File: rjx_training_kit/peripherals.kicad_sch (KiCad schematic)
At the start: 31 parts, among them Q7 BC817, Q8 BC817, SW3 SW_Push, U2 BME280, U3 DS3231M, U5 LIS3DH, U8 BQ27441-G1

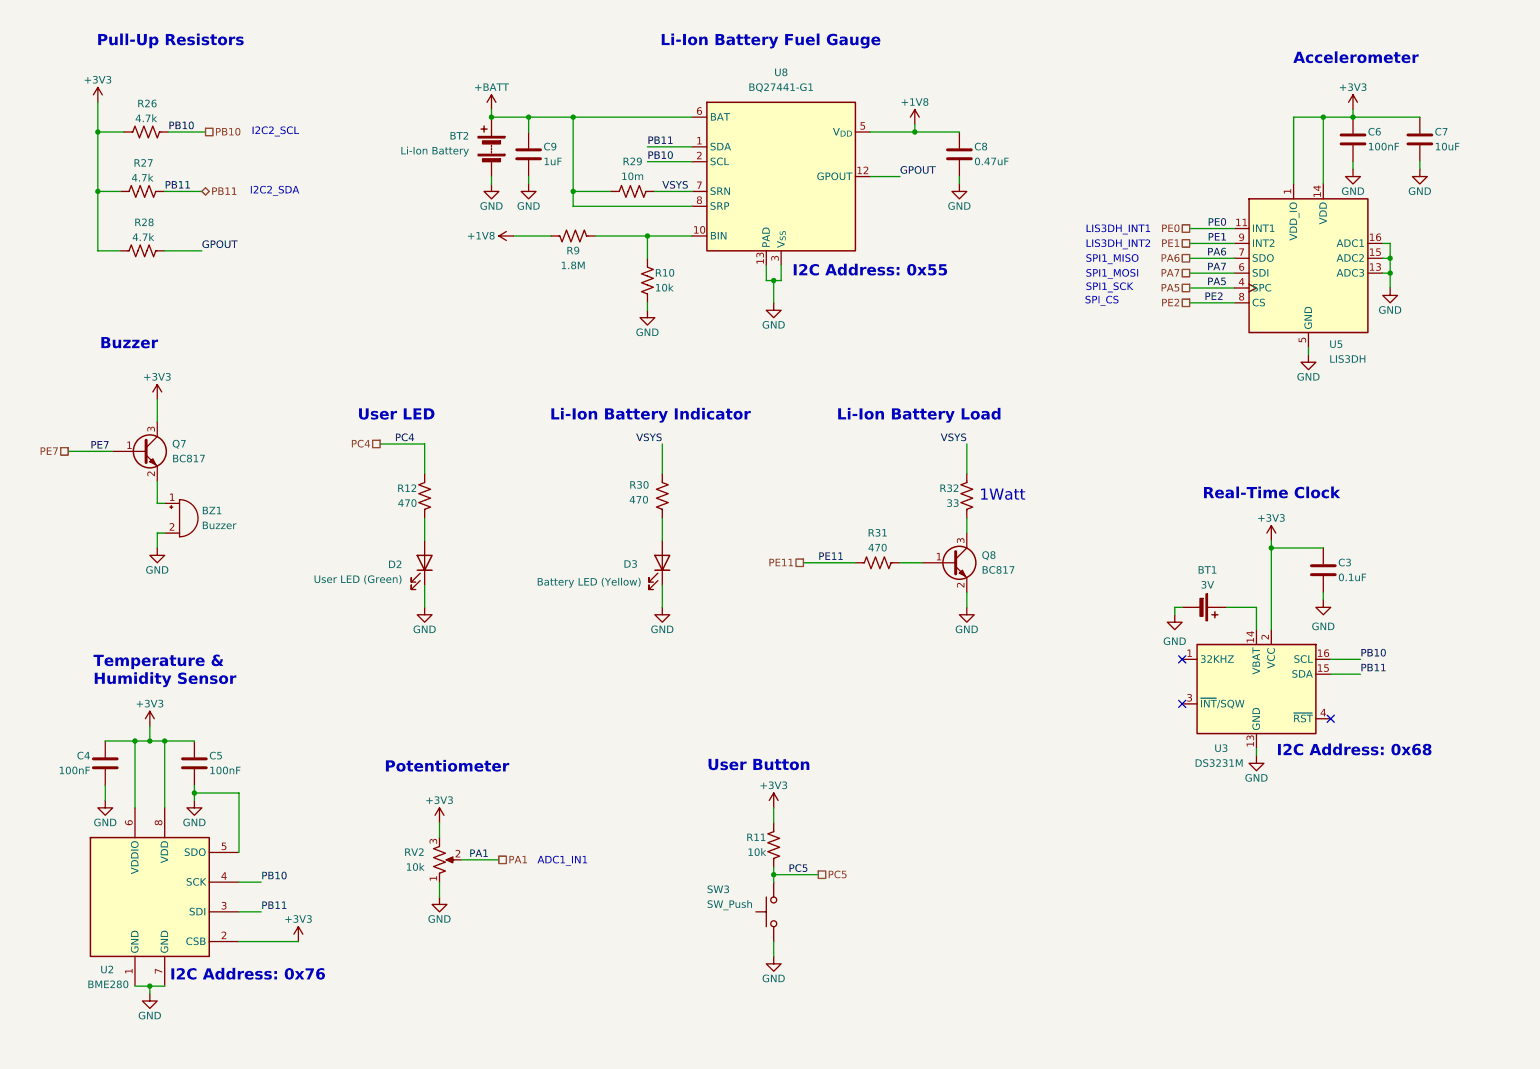
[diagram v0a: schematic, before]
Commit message: Update
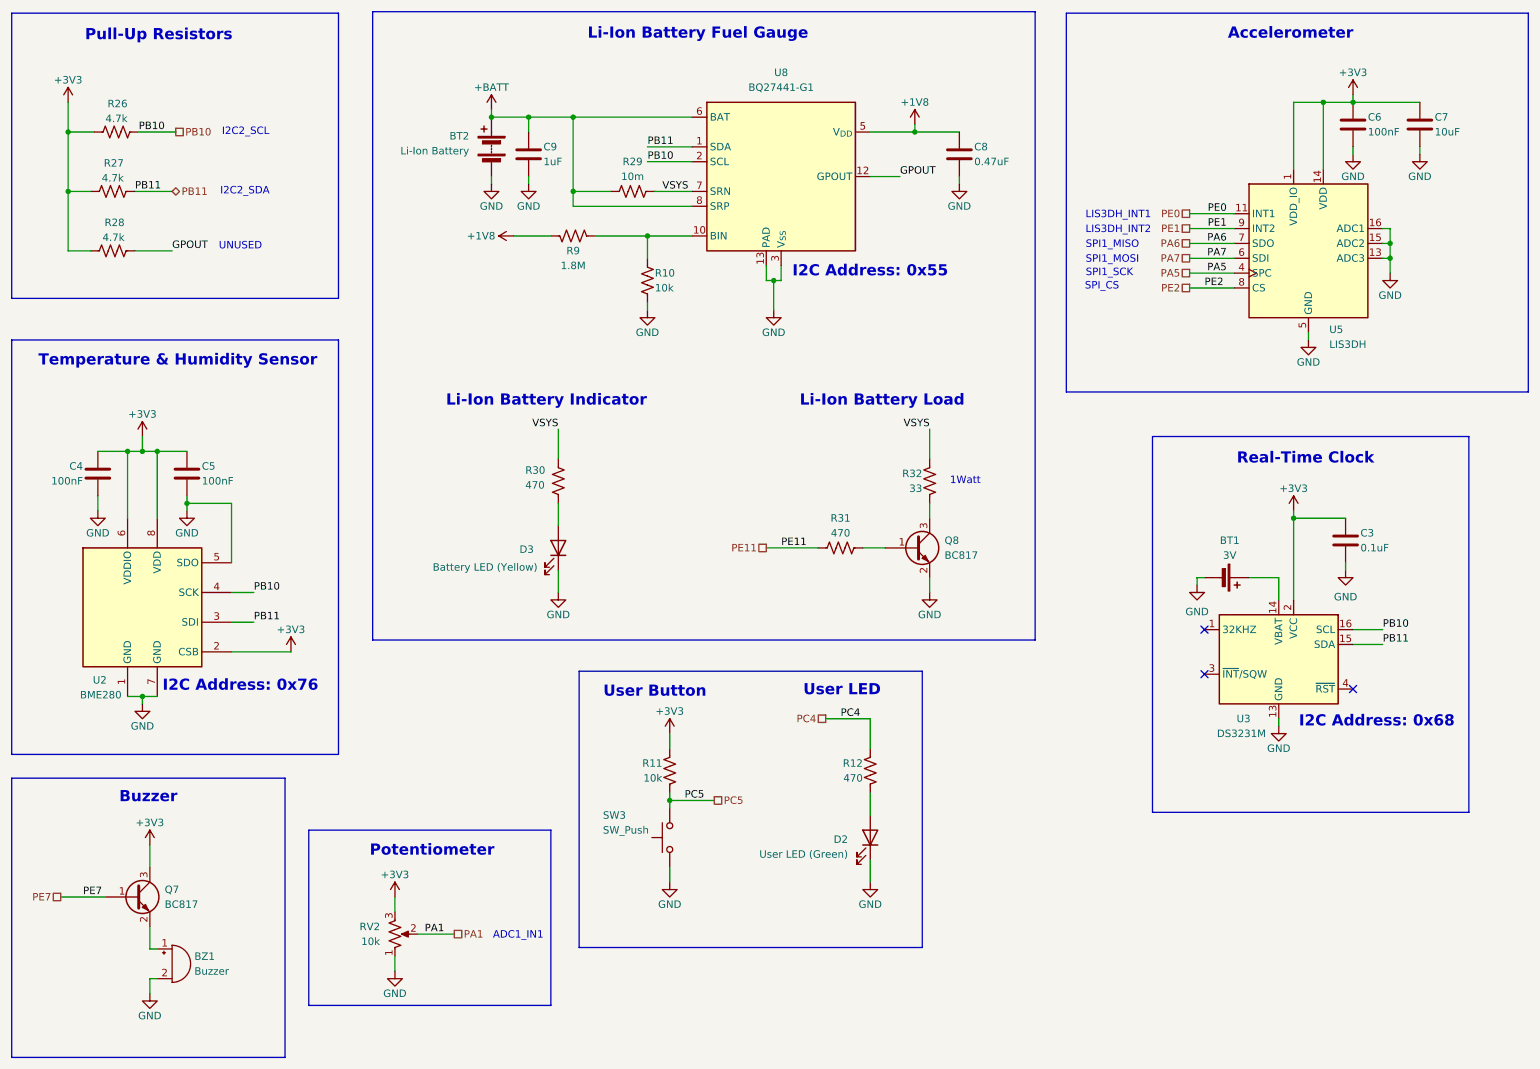
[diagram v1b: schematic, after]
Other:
- note added: "UNUSED"
- moved on the sheet: BT1, BZ1, C3, C4, C5, C6, C7, D2, D3, Q7, Q8, R11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
